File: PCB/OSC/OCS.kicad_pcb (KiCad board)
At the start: 2 copper layers, 46 x 33 mm, 45 parts, among them J1 Reset, J2 Wago, J3 TC2030-USB-NL-DS, J4 DC, J5 USB-C-Socket-H, J6 RELAY1, J7 RELAY2, SW1 SW_Push, SW2 SW_Reed, SW3 SW_Push, U1 ICS43434_MEMS_Mic, U3 Relay, U4 78L05, U6 ESP32-S3-MINI-1, U7 MD8942, U8 Relay, U9 VEML6040

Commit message: Images
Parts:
- removed REF**: Shadow, RevK:Shadow
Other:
- copper layers 2 -> 4

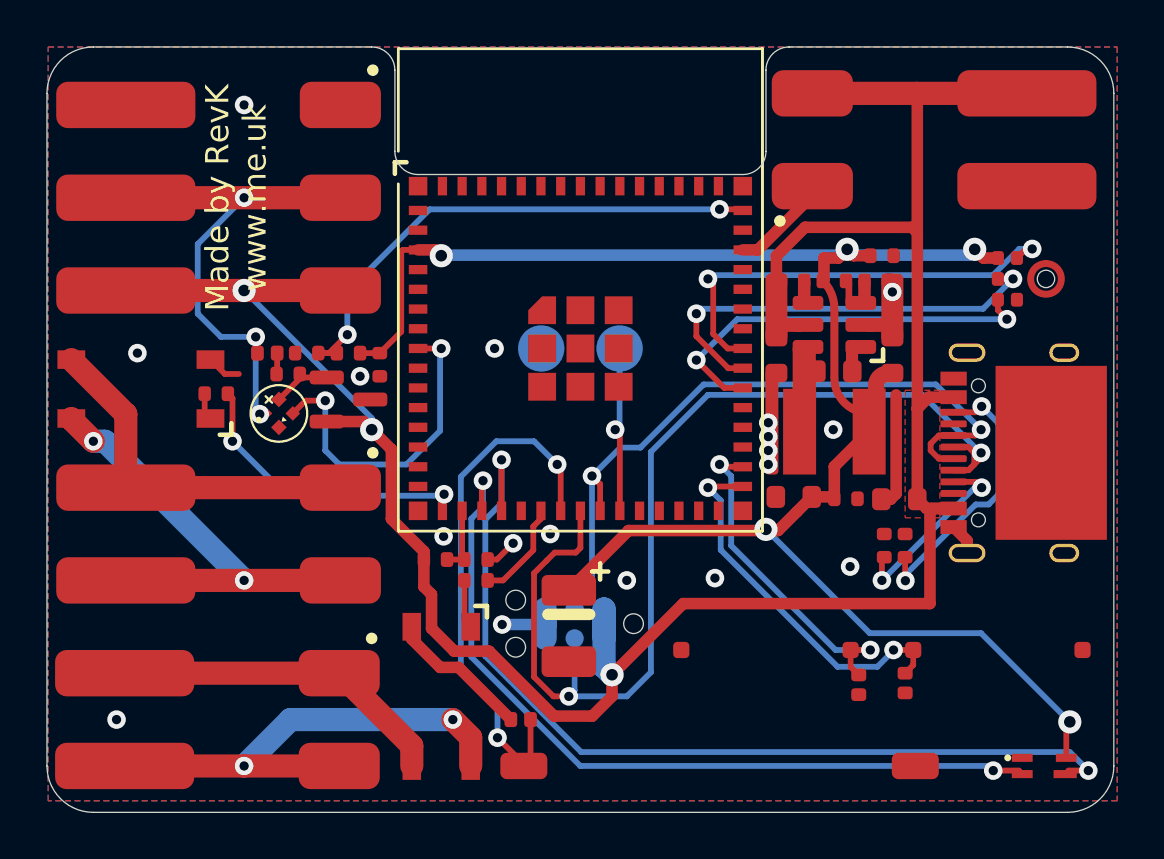
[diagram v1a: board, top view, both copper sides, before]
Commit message: PCB Update
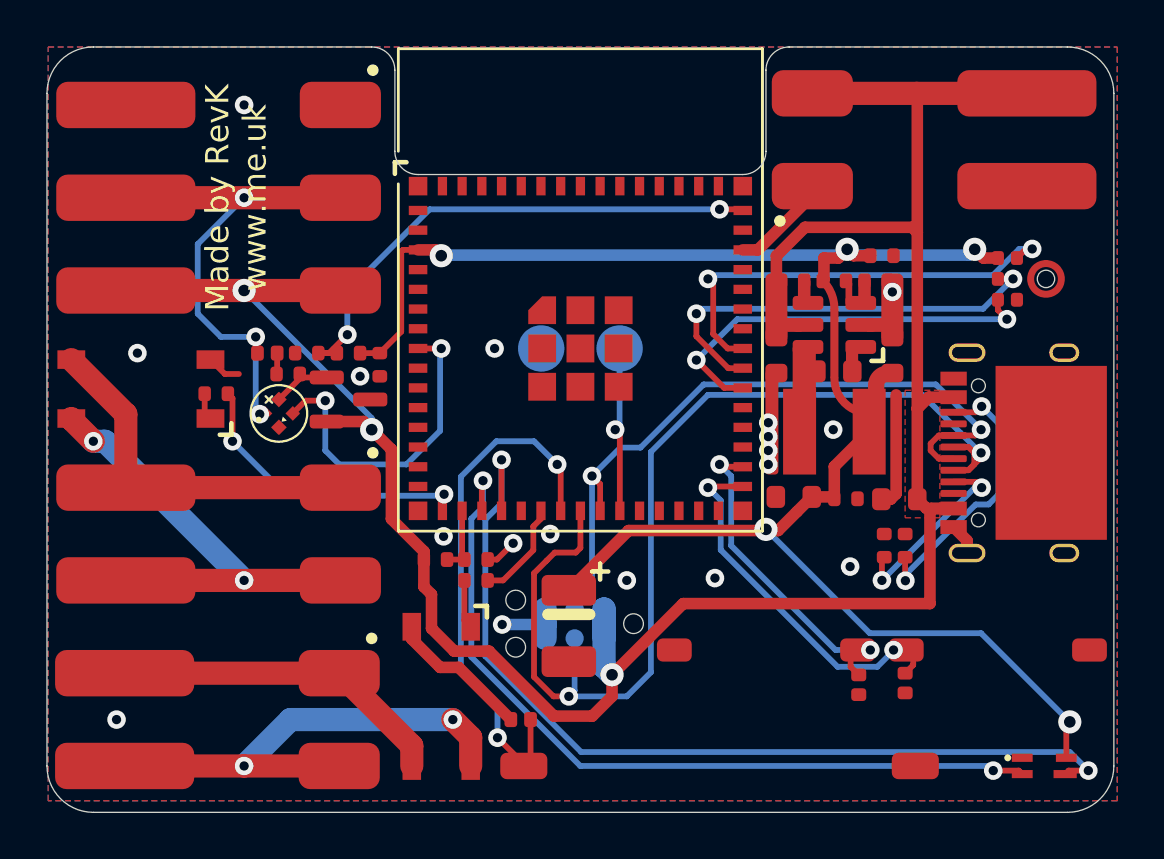
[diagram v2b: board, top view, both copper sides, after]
